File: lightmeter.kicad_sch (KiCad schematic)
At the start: 21 parts, among them J1 USB_C_Receptacle_USB2.0_16P, J2 5V input, J3 VEML 7700, J4 OLED Display, SW1 Value Rot, SW2 Setting Rot, SW3 BOOT, SW4 Shutter, U1 NCP1117-3.3_SOT223, U2 ESP32-S3-WROOM-1

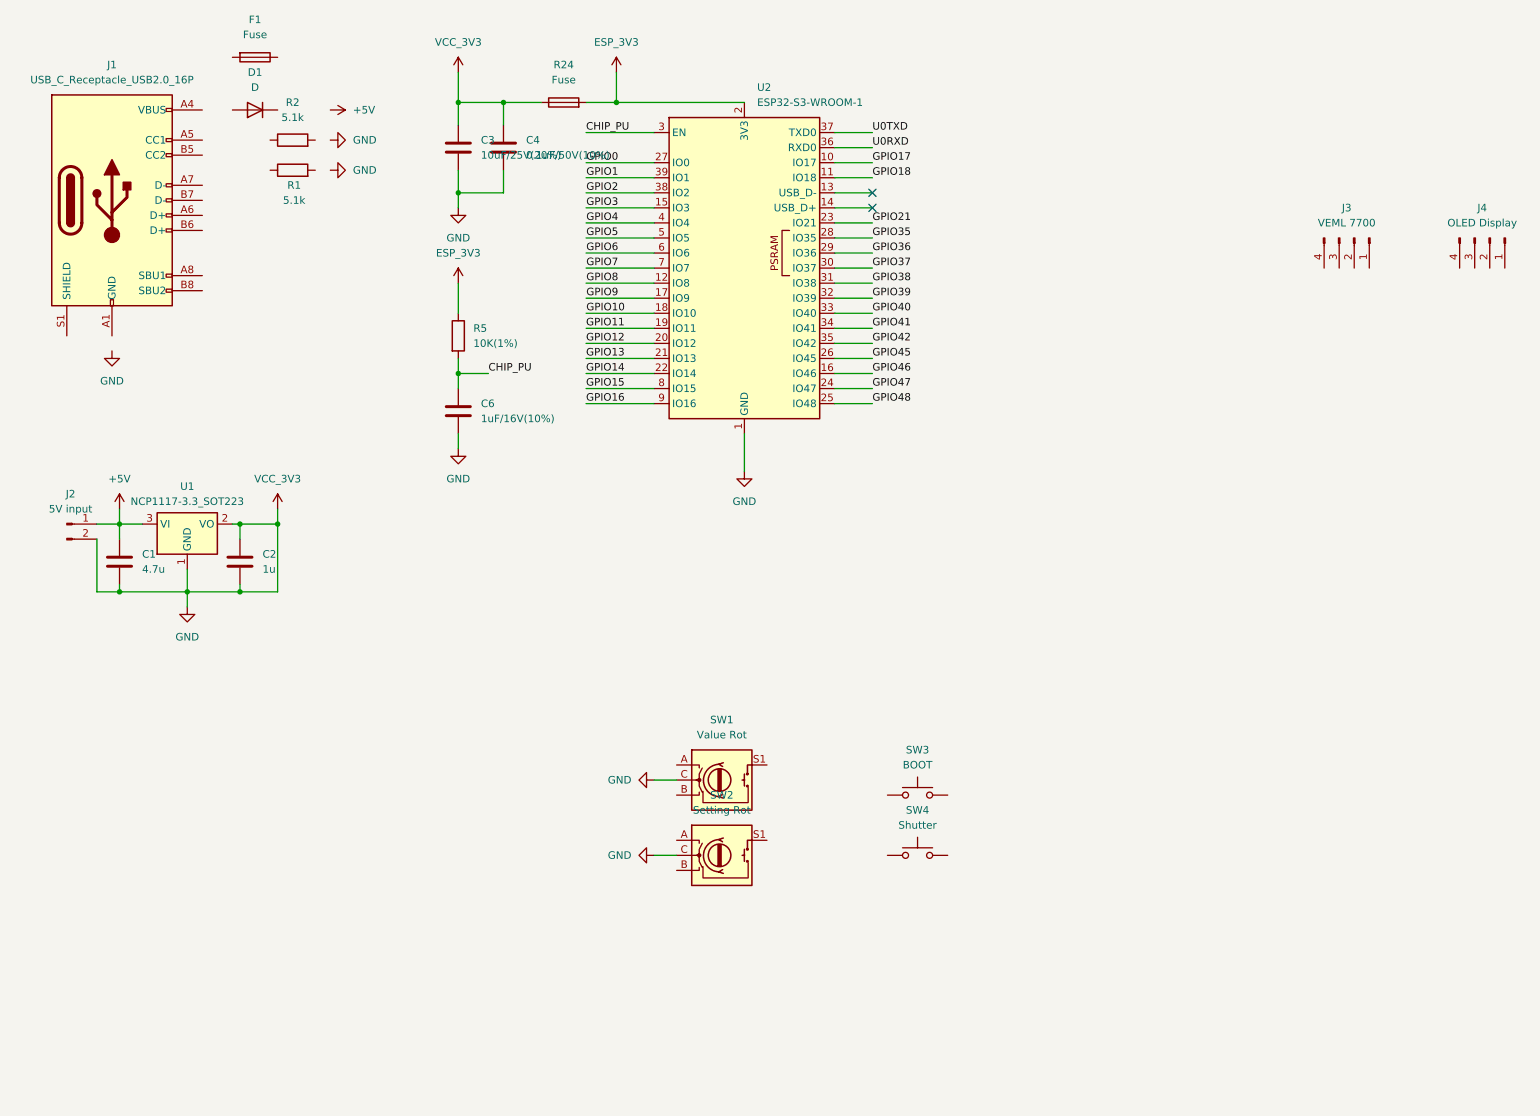
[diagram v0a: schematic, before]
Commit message: Finished schematic. Layout is next
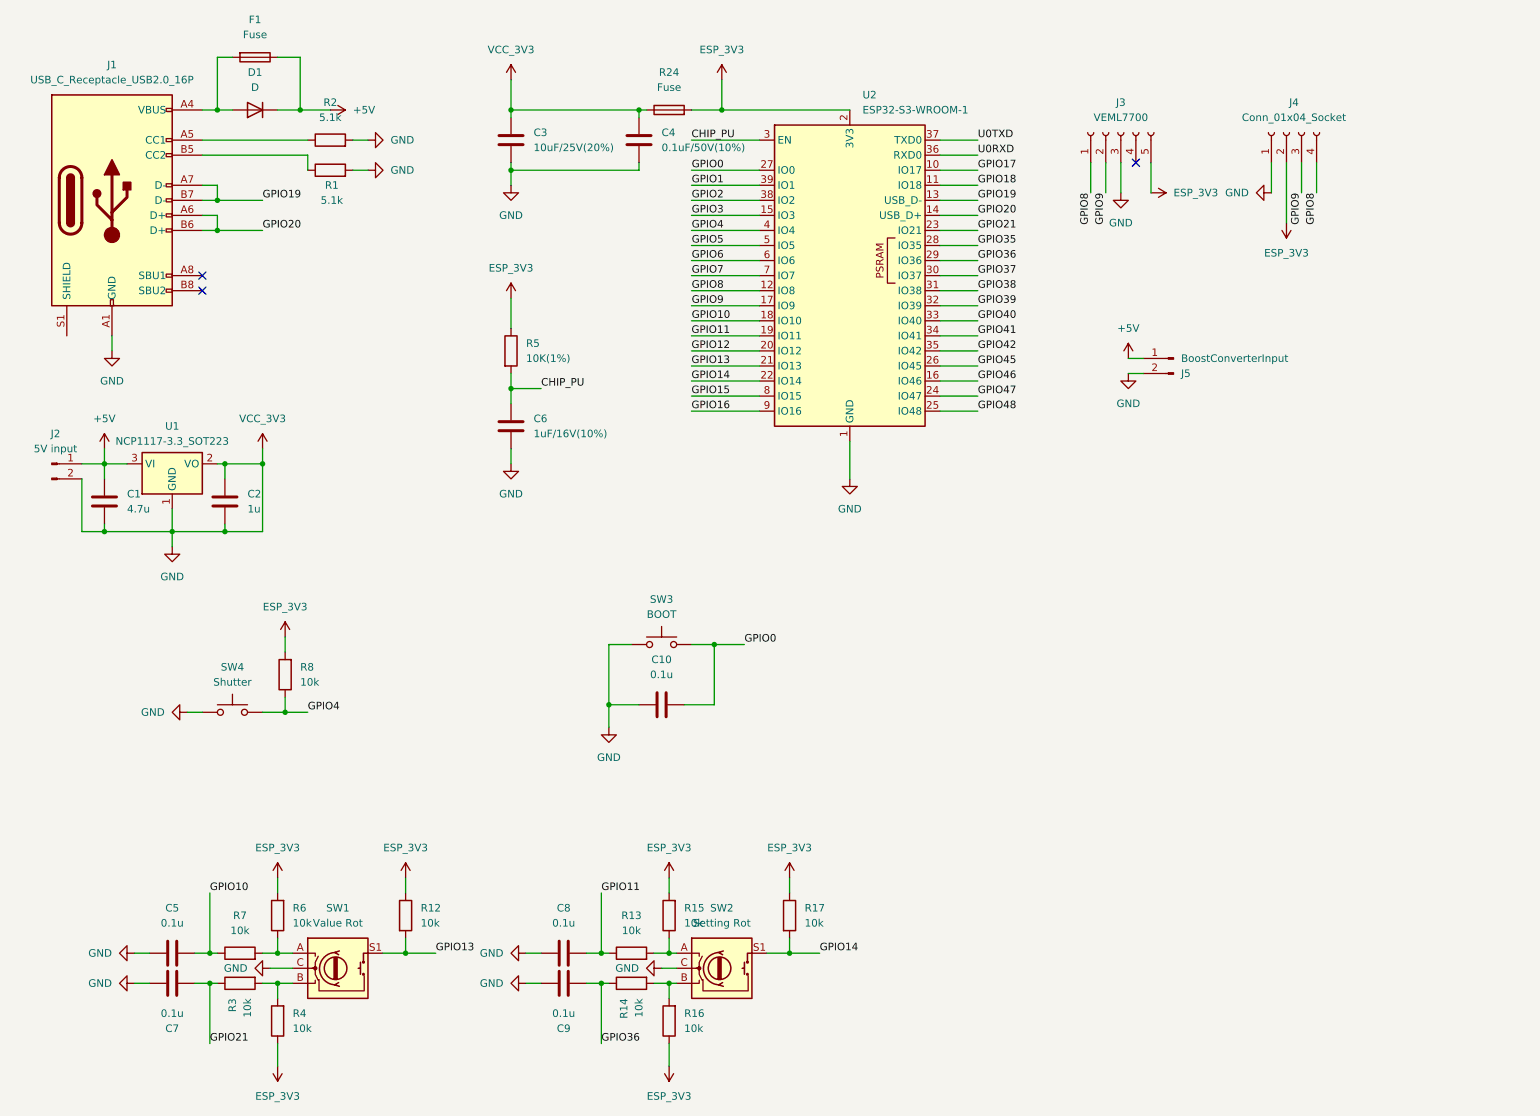
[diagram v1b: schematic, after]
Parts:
- removed J3: VEML 7700, symbol Connector:Conn_01x04_Pin
- removed J4: OLED Display, symbol Connector:Conn_01x04_Pin
- added C10, C5, C7, C8, C9: 0.1u, symbol Device:C
- added J3: VEML7700, symbol Connector:Conn_01x05_Socket
- added J4: Conn_01x04_Socket, symbol Connector:Conn_01x04_Socket
- added J5: BoostConverterInput, symbol Connector:Conn_01x02_Pin
- added R12, R13, R14, R15, R16, R17, R3, R4, R6, R7, R8: 10k, symbol Device:R
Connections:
- net +5V: now also D1.1 (K), F1.1, J5.1 (Pin_1)
- net ESP_3V3: now also J3.5 (Pin_5), J4.2 (Pin_2), R12.1, R15.2, R16.1, R17.1, R4.1, R6.2, R8.2
- net GND: now also J1.A1 (GND), J1.A12 (GND), J1.B1 (GND), J1.B12 (GND), R1.2, R2.2, SW3.1, SW4.1, C10.1, C5.1, C7.1, C8.1, C9.1, J3.3 (Pin_3), J4.1 (Pin_1), J5.2 (Pin_2)
- net GPIO0: now also SW3.2, C10.2
- net GPIO10: now also C5.2, R7.1
- net GPIO11: now also C8.2, R13.1
- net GPIO13: now also SW1.S1, R12.2
- net GPIO14: now also SW2.S1, R17.2
- net GPIO21: now also C7.2, R3.1
- net GPIO36: now also C9.2, R14.1
- net GPIO4: now also SW4.2, R8.1
- net GPIO8: now also J3.1 (Pin_1), J4.4 (Pin_4)
- net GPIO9: now also J3.2 (Pin_2), J4.3 (Pin_3)
- net GPIO19: now reaches U2.13 (USB_D-)
- net GPIO19: now also J1.A7 (D-), J1.B7 (D-)
- net GPIO20: now reaches U2.14 (USB_D+)
- net GPIO20: now also J1.A6 (D+), J1.B6 (D+)
- net at F1.2: now also D1.2 (A), J1.A4 (VBUS), J1.A9 (VBUS), J1.B4 (VBUS), J1.B9 (VBUS)
- net at SW1.A: now also R6.1, R7.2
- net at SW1.B: now also R3.2, R4.2
- net at J1.A5 (CC1): now also R2.1
- net at J1.B5 (CC2): now also R1.1
- net at SW2.A: now also R13.2, R15.1
- net at SW2.B: now also R14.2, R16.2
- no-connect marks 2 -> 3
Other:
- moved on the sheet: C1, C2, C3, C4, C6, J2, R1, R2, R24, R5, SW1, SW2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
